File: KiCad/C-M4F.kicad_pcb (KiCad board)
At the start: 2 copper layers, 100 x 100 mm, 258 parts, among them U1 PIN_STRIP_8, U2 PIN_STRIP_8, U3 PIN_STRIP_8, U31 PIN_STRIP_1, U32 PIN_STRIP_1, U33 PIN_STRIP_1, U34 PIN_STRIP_1, U35 PIN_STRIP_1, U36 PIN_STRIP_1, U37 PIN_STRIP_1, U38 PIN_STRIP_1, U4 PIN_STRIP_8, U41 PIN_STRIP_1, U42 PIN_STRIP_1, U43 PIN_STRIP_1, U44 PIN_STRIP_1, U45 PIN_STRIP_1, U46 PIN_STRIP_1, U47 PIN_STRIP_1, U48 PIN_STRIP_1

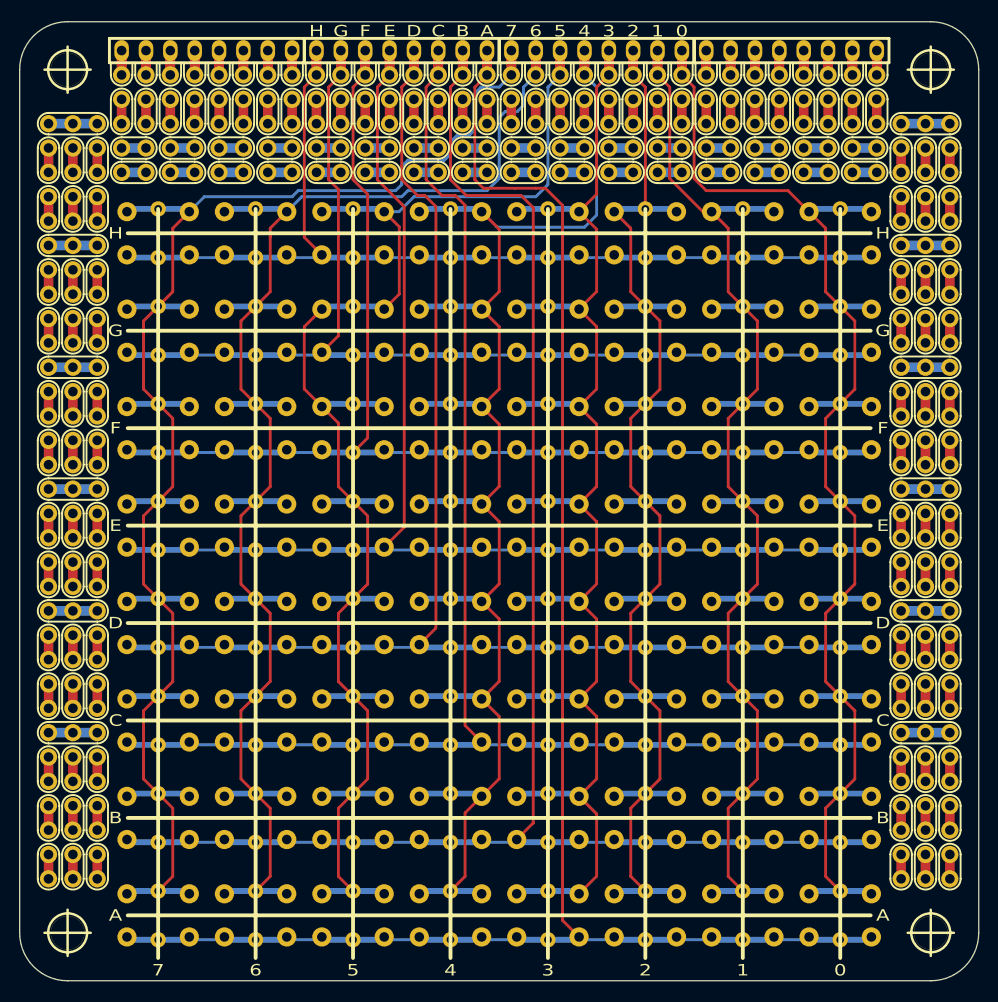
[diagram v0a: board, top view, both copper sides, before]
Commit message: initial PCB layout
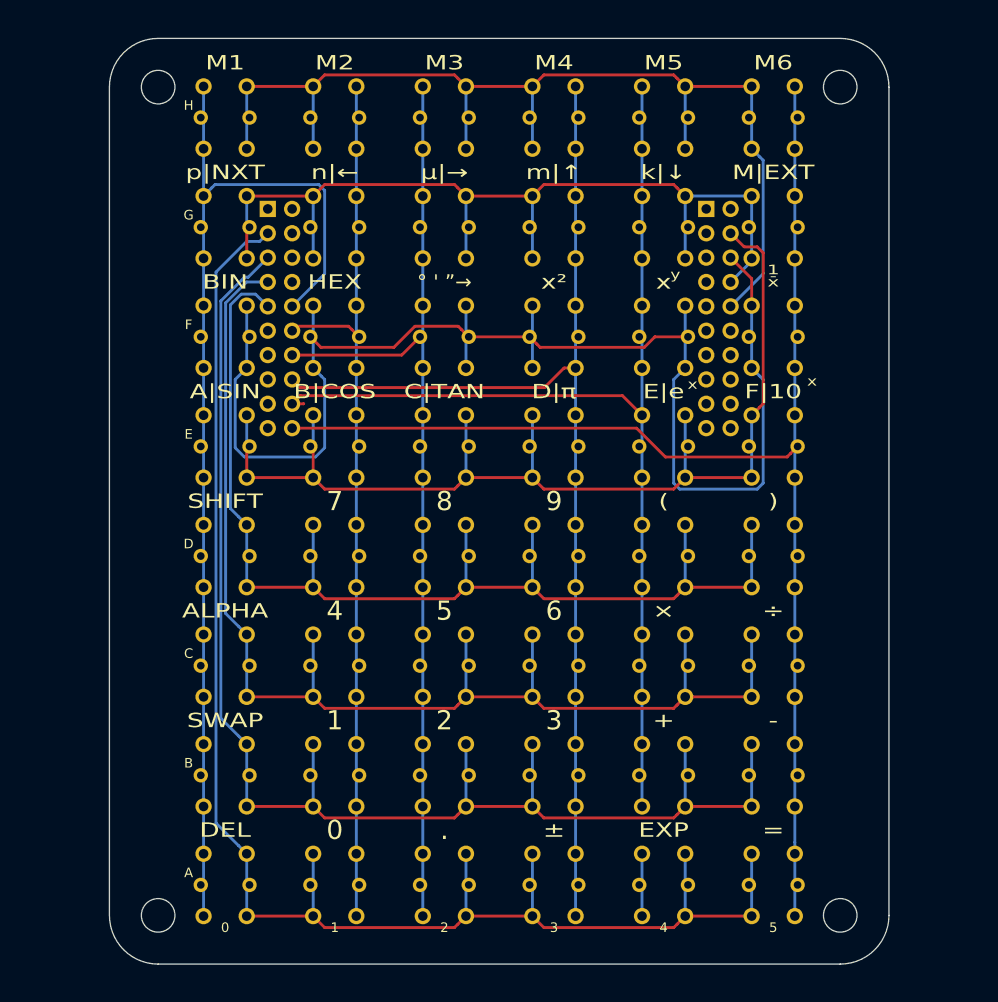
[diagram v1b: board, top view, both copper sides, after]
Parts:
- removed C0, C1, C2, C3, C4, C5, C6, C7, RA0, RB0, RC0, RD0, RE0, RF0, RG0, RH0, U31, U32, U33, U34, U35, U36, U37, U38, U41, U42, U43, U44, U45, U46, U47, U48: PIN_STRIP_1, C-M4F:Connected_Pad
- removed KEY_A6, KEY_A7, KEY_B6, KEY_B7, KEY_C6, KEY_C7, KEY_D6, KEY_D7, KEY_E6, KEY_E7, KEY_F6, KEY_F7, KEY_G6, KEY_G7, KEY_H6, KEY_H7: KEY, C-M4F:key
- removed REF** (x142): Double_Pad, C-M4F:Double_Pad
- removed REF** (x12): Triple_Pad, C-M4F:Triple_Pad
- removed U1, U2, U3, U4: PIN_STRIP_8, C-M4F:pin_strip_8
- removed hole_3mm5 (x4): VAL**, C-M4F:hole_3mm5
- added ?: MountingHole_3.5mm, Mounting_Holes:MountingHole_3.5mm, F.Cu at (140.6, 101.8)
- added ?: MountingHole_3.5mm, Mounting_Holes:MountingHole_3.5mm, F.Cu at (69.4, 188.2)
- added ?: MountingHole_3.5mm, Mounting_Holes:MountingHole_3.5mm, F.Cu at (140.6, 188.2)
- added ?: MountingHole_3.5mm, Mounting_Holes:MountingHole_3.5mm, F.Cu at (69.4, 101.8)
- added G***: LOGO, C-M4F:Logo_silk_CC-BY-SA_10x4.5mm, B.Cu at (141.2, 129.8)
- added J_1AB1: BoosterPackXL_AB, C-M4F:BoosterPackXL_AB, B.Cu at (80.9, 114.5)
- added J_1CD1: BoosterPackXL_CD, C-M4F:BoosterPackXL_CD, B.Cu at (126.6, 114.5)
- moved KEY_H0 65.3 mm to (76.4, 105.0), turned to 180 degrees
- moved KEY_G0 65.0 mm to (76.4, 116.4), turned to 180 degrees
- moved KEY_F0 64.8 mm to (76.4, 127.9), turned to 180 degrees
- moved KEY_E0 64.7 mm to (76.4, 139.3), turned to 180 degrees
- moved KEY_D0 64.5 mm to (76.4, 150.7), turned to 180 degrees
- moved KEY_C0 64.4 mm to (76.4, 162.1), turned to 180 degrees
- moved KEY_B0 64.3 mm to (76.4, 173.6), turned to 180 degrees
- moved KEY_A0 64.2 mm to (76.4, 185.0), turned to 180 degrees
- moved KEY_H5 45.4 mm to (133.6, 105.0), turned to 0 degrees
- moved KEY_G5 45.1 mm to (133.6, 116.4), turned to 0 degrees
- moved KEY_F5 44.8 mm to (133.6, 127.9), turned to 0 degrees
- moved KEY_E5 44.6 mm to (133.6, 139.3), turned to 0 degrees
- moved KEY_D5 44.4 mm to (133.6, 150.7), turned to 0 degrees
- moved KEY_H1 44.2 mm to (87.9, 105.0), turned to 0 degrees
- moved KEY_C5 44.2 mm to (133.6, 162.1), turned to 0 degrees
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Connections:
- net /KEYPAD_COL_0 renamed KEY_COLUMN_0
- net /KEYPAD_COL_1 renamed KEY_COLUMN_1
- net /KEYPAD_COL_2 renamed KEY_COLUMN_2
- net /KEYPAD_COL_3 renamed KEY_COLUMN_3
- net /KEYPAD_COL_4 renamed KEY_COLUMN_4
- net /KEYPAD_COL_5 renamed KEY_COLUMN_5
- net /KEYPAD_ROW_A renamed KEY_ROW_A
- net /KEYPAD_ROW_B renamed KEY_ROW_B
- net /KEYPAD_ROW_C renamed KEY_ROW_C
- net /KEYPAD_ROW_D renamed KEY_ROW_D
- net /KEYPAD_ROW_E renamed KEY_ROW_E
- net /KEYPAD_ROW_F renamed KEY_ROW_F
- net /KEYPAD_ROW_G renamed KEY_ROW_G
- net /KEYPAD_ROW_H renamed KEY_ROW_H
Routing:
- net /KEYPAD_COL_7: track 179.8 -> 0.00 mm
- net /KEYPAD_COL_6: track 172.9 -> 0.00 mm
- net KEY_ROW_D: track 190.1 -> 123.6 mm
- net KEY_ROW_B: track 215.5 -> 149.2 mm
- net KEY_ROW_C: track 200.9 -> 135.9 mm
- net KEY_ROW_A: track 226.3 -> 164.1 mm
- net KEY_ROW_E: track 179.4 -> 117.6 mm
- net KEY_ROW_G: track 158.2 -> 98.9 mm
- net KEY_COLUMN_1: track 152.4 -> 96.1 mm
- net KEY_COLUMN_2: track 150.7 -> 102.6 mm
- net KEY_COLUMN_0: track 161.0 -> 115.3 mm
- net KEY_COLUMN_4: track 166.1 -> 122.4 mm
- net KEY_COLUMN_3: track 153.7 -> 119.2 mm
- net KEY_ROW_H: track 147.6 -> 113.4 mm
- net KEY_COLUMN_5: track 166.7 -> 142.8 mm
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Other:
- board size 100 x 100 mm -> 81.3 x 96.5 mm
- board text added: "("
- board text added: ")"
- board text added: "+"
- board text added: "-"
- board text added: "."
- board text added: "8"
- board text added: "9"
- board text added: "="
- board text added: "ALPHA"
- board text added: "A|SIN"
- board text added: "BIN"
- board text added: "B|COS"
- board text added: "C|TAN"
- board text added: "DEL"
- board text added: "Dirk Heisswolf 2019"
- board text added: "D|π"
- board text added: "EXP"
- board text added: "E|e"
- board text added: "F|10"
- board text added: "HEX"
- board text added: "M1"
- board text added: "M2"
- board text added: "M3"
- board text added: "M4"
- board text added: "M5"
- board text added: "M6"
- board text added: "M|EXT"
- board text added: "RevA"
- board text added: "SHIFT"
- board text added: "SWAP"
- board text added: "k|↓"
- board text added: "m|↑"
- board text added: "n|←"
- board text added: "p|NXT"
- board text added: "x"
- board text added: "x²"
- board text added: "y"
- board text added: "° ' ”→"
- board text added: "±"
- board text added: "×"
- board text added: "÷"
- board text added: "μ|→"
- board text removed: "CC BY-SA"
- board text removed: "Dirk Heisswolf 2017"
